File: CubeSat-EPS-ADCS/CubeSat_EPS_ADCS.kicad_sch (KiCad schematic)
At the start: 18 parts, among them J1 Conn_01x02_Pin, J2 Conn_01x03_Pin, J3 Conn_01x08_Pin, J4 Conn_01x02_Pin, J5 Screw_Terminal_01x02, J6 Screw_Terminal_01x02, J7 Screw_Terminal_01x02, U1 DRV8833 Module, U2 DRV8833 Module, U4 Buck_LM2596

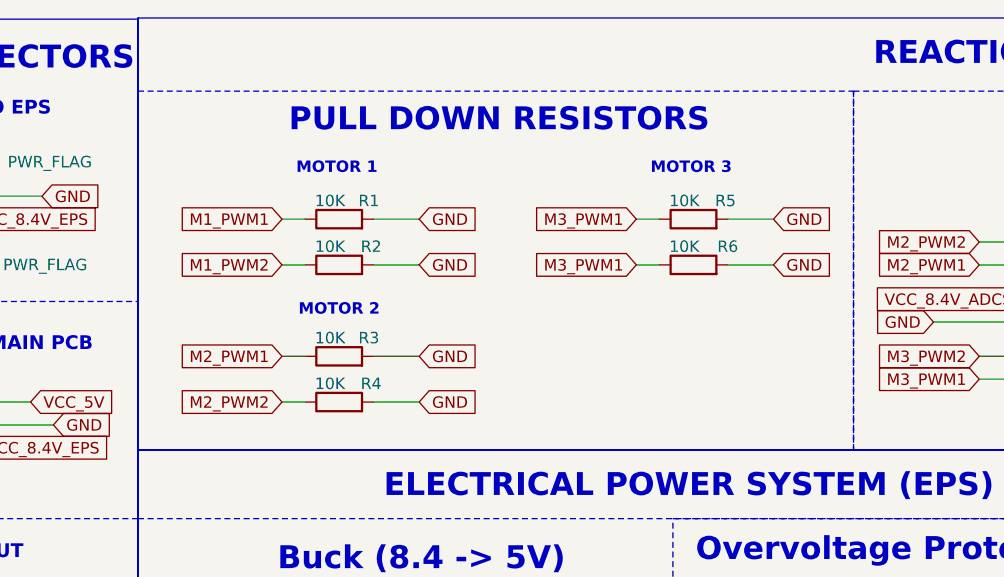
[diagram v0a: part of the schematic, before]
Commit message: Mostly fine tuning the boards, also added capacitor for battery ADC
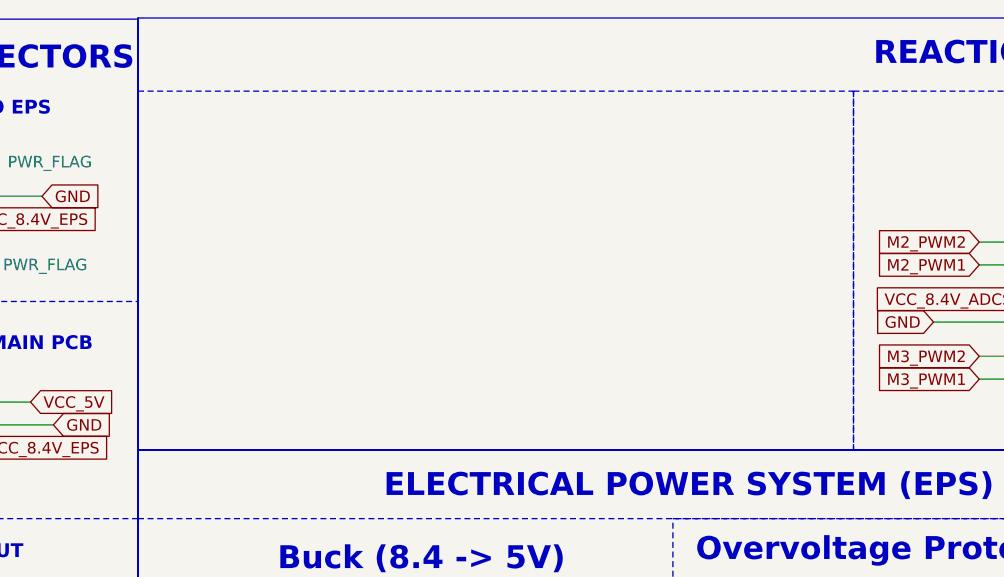
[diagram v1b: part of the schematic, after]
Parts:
- removed R1, R2, R3, R4, R5, R6: 10K, Resistor_THT:R_Axial_DIN0207_L6.3mm_D2.5mm_P7.62mm_Horizontal, symbol Device:R
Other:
- note removed: "PULL DOWN RESISTORS"
